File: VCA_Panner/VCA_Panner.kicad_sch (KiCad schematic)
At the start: 40 parts, among them J1 CV1, J2 Ch1_in, J3 Ch1_out, J4 CV2, J5 Ch2_in, J6 Ch2_out, SW1 SW_DPDT_x2, SW2 SW_DPDT_x2, U1 TL074, U2 AS3360, U3 TL072

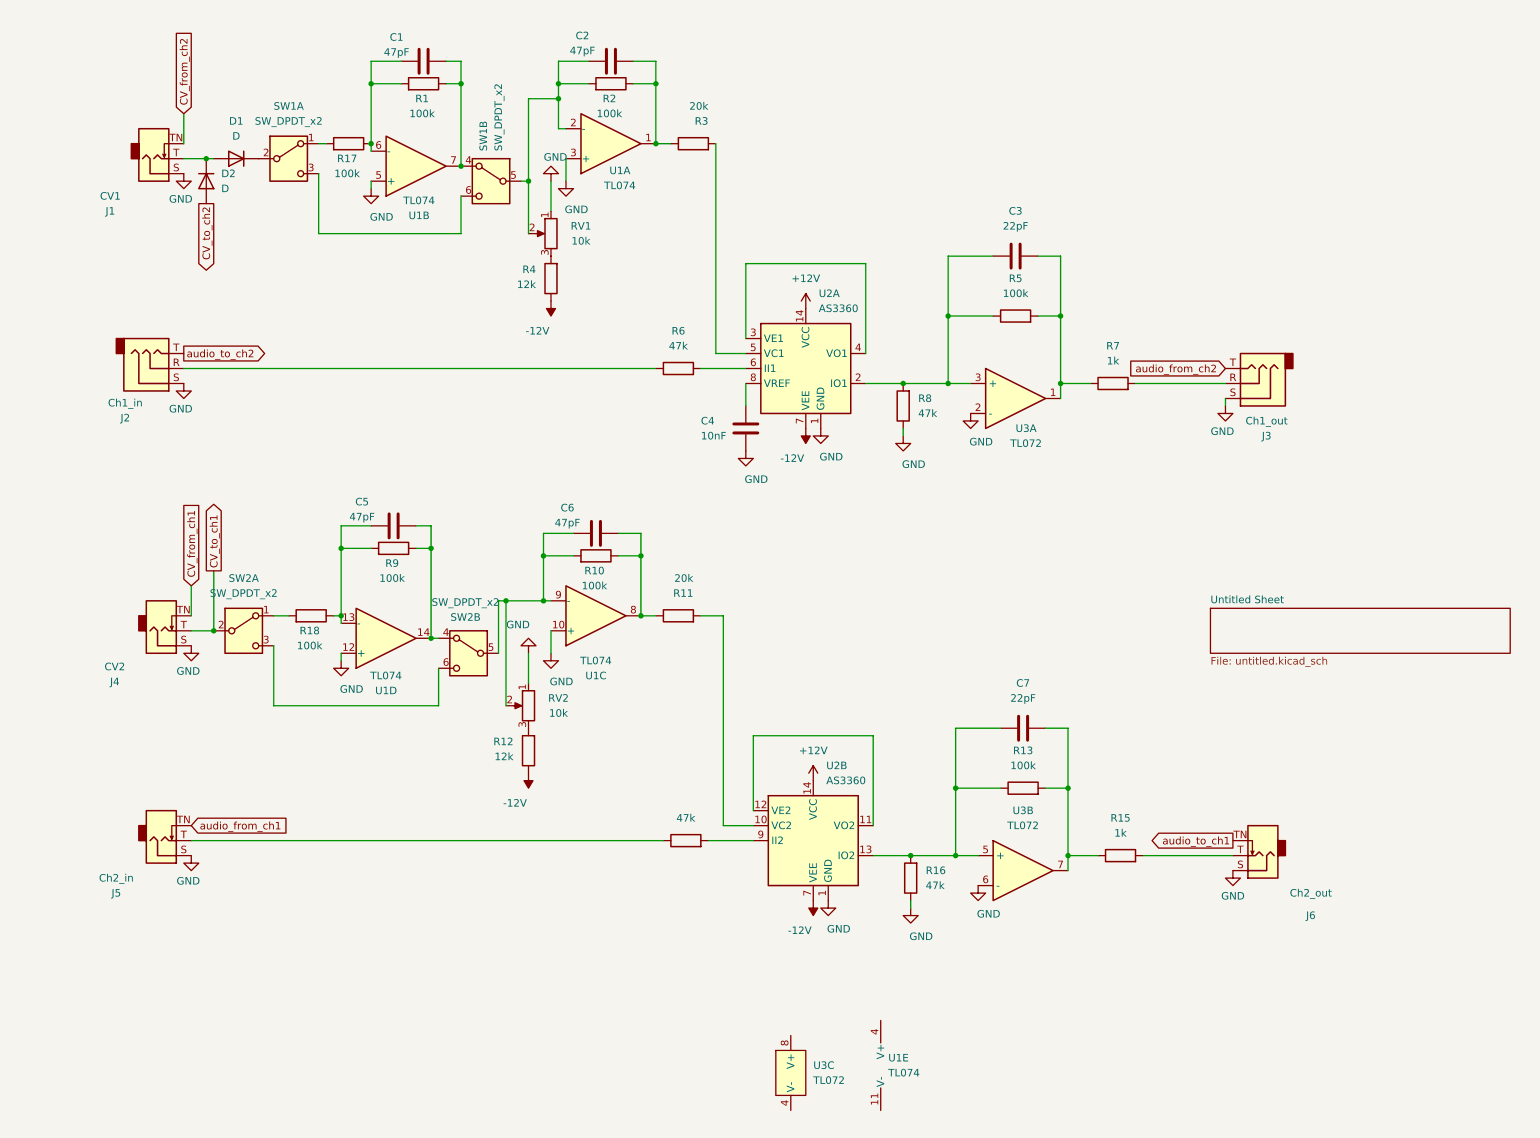
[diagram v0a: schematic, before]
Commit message: feitw bugfixes
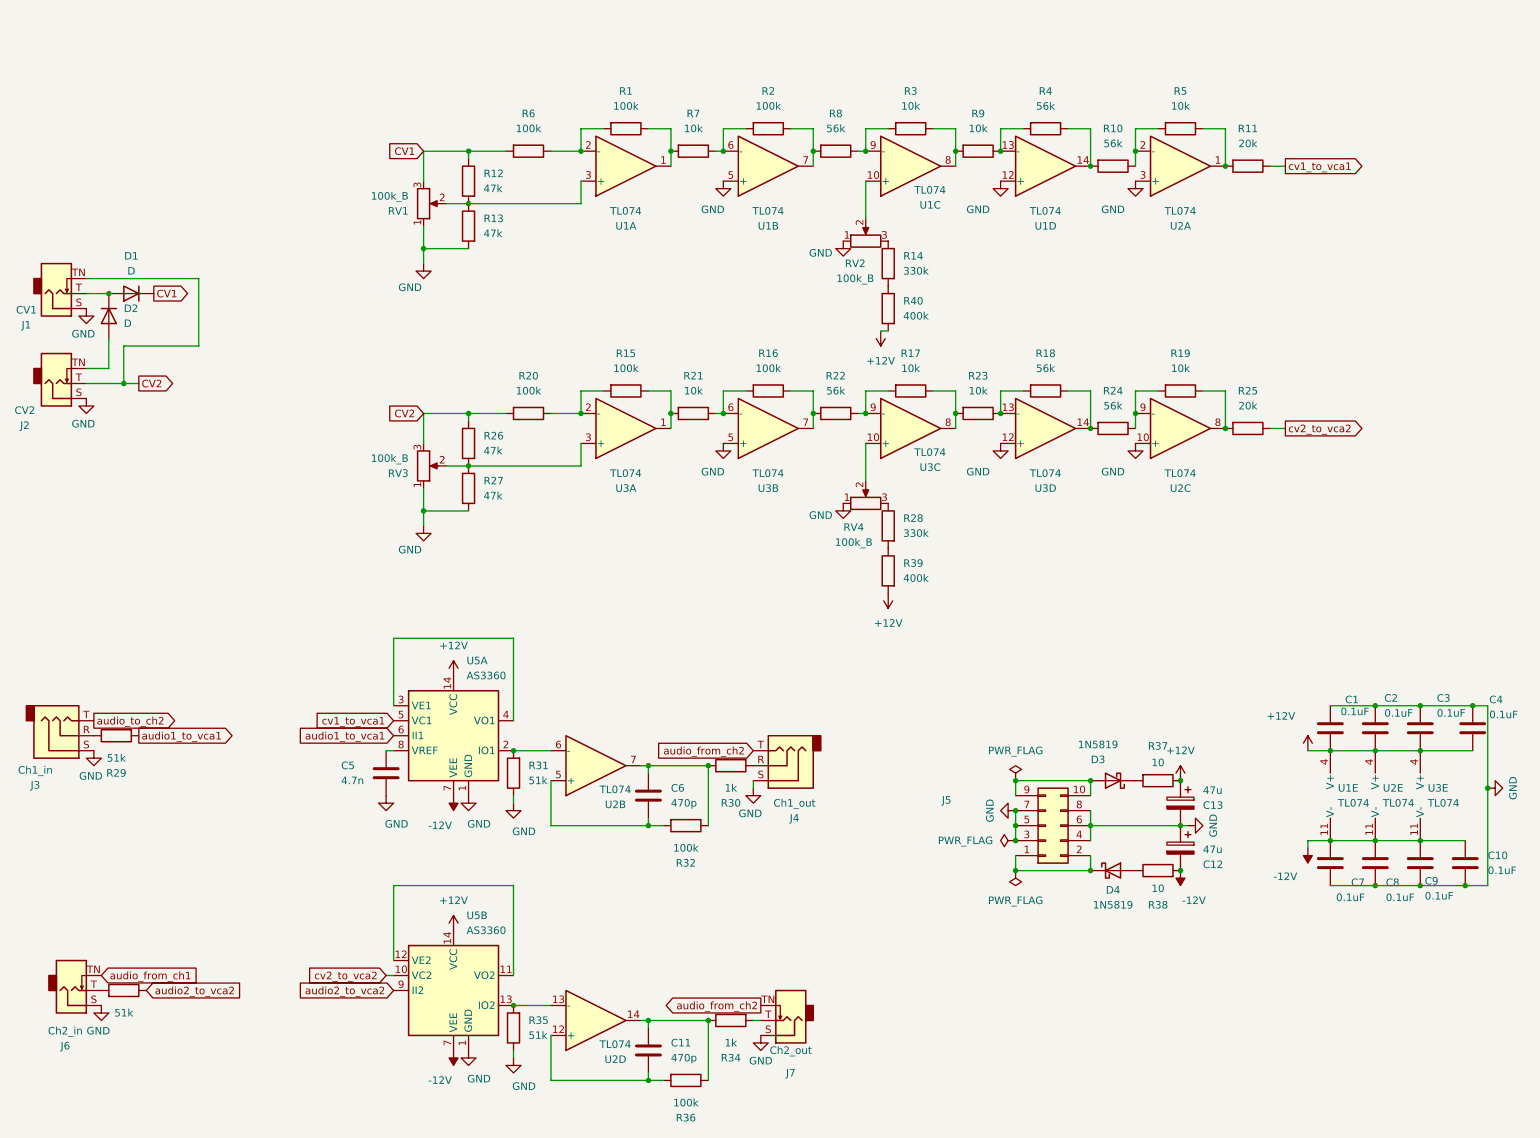
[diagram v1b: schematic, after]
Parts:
- removed C5: 47pF, symbol Device:C
- removed SW1, SW2: SW_DPDT_x2, symbol Switch:SW_DPDT_x2
- removed U3: TL072, 4ms_Package_SSOP:TSSOP-8_4.4x3mm_Pitch0.65mm, symbol PCM_4ms_IC:TL072
- added C10, C4, C8, C9: 0.1uF, Capacitor_SMD:C_0805_2012Metric_Pad1.18x1.45mm_HandSolder, symbol Device:C
- added C11: 470p, Capacitor_SMD:C_0805_2012Metric_Pad1.18x1.45mm_HandSolder, symbol Device:C
- added C12, C13: 47u, Capacitor_THT:CP_Radial_D4.0mm_P2.00mm, symbol Device:C_Polarized
- added D3, D4: 1N5819, Diode_THT:D_DO-41_SOD81_P2.54mm_Vertical_AnodeUp, symbol Diode:1N5819
- added J5: ~, mort_mix:Pins_2x05_2.54mm_TH_Europower_shrouded, symbol Connector_Generic:Conn_02x05_Odd_Even
- added R19, R21, R23, R7: 10k, Resistor_SMD:R_0805_2012Metric_Pad1.20x1.40mm_HandSolder, symbol Device:R
- added R20, R32, R36: 100k, Resistor_SMD:R_0805_2012Metric_Pad1.20x1.40mm_HandSolder, symbol Device:R
- added R22, R24, R8: 56k, Resistor_SMD:R_0805_2012Metric_Pad1.20x1.40mm_HandSolder, symbol Device:R
- added R25: 20k, Resistor_SMD:R_0805_2012Metric_Pad1.20x1.40mm_HandSolder, symbol Device:R
- added R26, R27: 47k, Resistor_SMD:R_0805_2012Metric_Pad1.20x1.40mm_HandSolder, symbol Device:R
- added R28: 330k, Resistor_SMD:R_0805_2012Metric_Pad1.20x1.40mm_HandSolder, symbol Device:R
- added R29, R33, R35: 51k, Resistor_SMD:R_0805_2012Metric_Pad1.20x1.40mm_HandSolder, symbol Device:R
- added R34: 1k, Resistor_SMD:R_0805_2012Metric_Pad1.20x1.40mm_HandSolder, symbol Device:R
- added R37, R38: 10, Resistor_SMD:R_0805_2012Metric_Pad1.20x1.40mm_HandSolder, symbol Device:R
- added R39, R40: 400k, Resistor_SMD:R_0805_2012Metric_Pad1.20x1.40mm_HandSolder, symbol Device:R
- added RV3, RV4: 100k_B, mort_mix:Potentiometer_Alpha_RD901F-40-00D_Single_Vertical_withhole, symbol Device:R_Potentiometer
- added U2, U3: TL074, Package_SO:SO-14_3.9x8.65mm_P1.27mm, symbol Amplifier_Operational:TL074
- C1, C2: value 47pF -> 0.1uF; footprint (none) -> Capacitor_SMD:C_0805_2012Metric_Pad1.18x1.45mm_HandSolder
- C3, C7: value 22pF -> 0.1uF; footprint (none) -> Capacitor_SMD:C_0805_2012Metric_Pad1.18x1.45mm_HandSolder
- C5: renamed from C4; value 10nF -> 4.7n; footprint (none) -> Capacitor_SMD:C_0805_2012Metric_Pad1.18x1.45mm_HandSolder
- C6: value 47pF -> 470p; footprint (none) -> Capacitor_SMD:C_0805_2012Metric_Pad1.18x1.45mm_HandSolder
- D1, D2: footprint (none) -> Diode_SMD:D_0805_2012Metric_Pad1.15x1.40mm_HandSolder
- J1: footprint (none) -> mort_mix:PJ398SM
- J2: renamed from J4; footprint (none) -> mort_mix:PJ398SM
- J3: renamed from J2; footprint (none) -> mort_mix:Jack_3.5mm_QingPu_WQP-PJ366ST_Vertical
- J4: renamed from J3; footprint (none) -> mort_mix:Jack_3.5mm_QingPu_WQP-PJ366ST_Vertical
- J6: renamed from J5; footprint (none) -> mort_mix:PJ398SM
- J7: renamed from J6; footprint (none) -> mort_mix:PJ398SM
- R1, R11, R2: footprint (none) -> Resistor_SMD:R_0805_2012Metric_Pad1.20x1.40mm_HandSolder
- R10, R18: value 100k -> 56k; footprint (none) -> Resistor_SMD:R_0805_2012Metric_Pad1.20x1.40mm_HandSolder
- R12: value 12k -> 47k; footprint (none) -> Resistor_SMD:R_0805_2012Metric_Pad1.20x1.40mm_HandSolder
- R13: value 100k -> 47k; footprint (none) -> Resistor_SMD:R_0805_2012Metric_Pad1.20x1.40mm_HandSolder
- R14: value 47k -> 330k; footprint (none) -> Resistor_SMD:R_0805_2012Metric_Pad1.20x1.40mm_HandSolder
- R15: value 1k -> 100k; footprint (none) -> Resistor_SMD:R_0805_2012Metric_Pad1.20x1.40mm_HandSolder
- R16, R6: value 47k -> 100k; footprint (none) -> Resistor_SMD:R_0805_2012Metric_Pad1.20x1.40mm_HandSolder
- R17, R5, R9: value 100k -> 10k; footprint (none) -> Resistor_SMD:R_0805_2012Metric_Pad1.20x1.40mm_HandSolder
- R3: value 20k -> 10k; footprint (none) -> Resistor_SMD:R_0805_2012Metric_Pad1.20x1.40mm_HandSolder
- R30: renamed from R7; footprint (none) -> Resistor_SMD:R_0805_2012Metric_Pad1.20x1.40mm_HandSolder
- R31: renamed from R8; value 47k -> 51k; footprint (none) -> Resistor_SMD:R_0805_2012Metric_Pad1.20x1.40mm_HandSolder
- R4: value 12k -> 56k; footprint (none) -> Resistor_SMD:R_0805_2012Metric_Pad1.20x1.40mm_HandSolder
- RV1, RV2: value 10k -> 100k_B; footprint (none) -> mort_mix:Potentiometer_Alpha_RD901F-40-00D_Single_Vertical_withhole
- U1: footprint (none) -> Package_SO:SO-14_3.9x8.65mm_P1.27mm
- U5: renamed from U2; footprint (none) -> Package_SO:SOIC-16_3.9x9.9mm_P1.27mm
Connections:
- net CV_to_ch1 is gone; now on net CV2: J2.T
- net CV_to_ch2 is gone; now on an unnamed net: D2.2 (A)
- net audio_to_ch1 is gone; now on net audio_from_ch2: J7.TN
- net +12V: now also C1.1, C2.1, C3.1, U1.4 (V+), C13.1, C4.2, R37.1, R39.2, R40.2, U2.4 (V+), U3.4 (V+)
- net -12V: now also C7.2, U1.11 (V-), C10.2, C12.2, C8.2, C9.2, R38.2, U2.11 (V-), U3.11 (V-); no longer R12.1, R4.1
- net GND: now also C1.2, C2.2, C3.2, C7.1, R13.2, C10.1, C12.1, C13.2, C4.1, C8.1, C9.1, J5.3 (Pin_3), J5.4 (Pin_4), J5.5 (Pin_5), J5.6 (Pin_6), J5.7 (Pin_7), J5.8 (Pin_8), R27.2, R35.1, RV3.1, RV4.1, U2.10 (+), U2.3 (+), U3.12 (+), U3.5 (+); no longer R16.1, U1.10 (+), U1.3 (+)
- net at R31.2, U5.2 (IO1): now also U2.6 (-); no longer C3.1, R5.1
- net CV1: now reaches D1.1 (K)
- net CV1: now also R12.1, R6.2, RV1.3
- net at R12.2: now also R13.1, RV1.2, U1.3 (+); no longer RV2.3
- net at R18.2: now also R23.1, U3.13 (-)
- net at R14.1: now also RV2.3; no longer J6.T
- net at R6.1: now also R1.2, U1.2 (-); no longer J3.R
- net audio1_to_vca1: now reaches U5.6 (II1)
- net audio1_to_vca1: now also R29.2; no longer R6.2
- net at R11.2: now also R5.1, U2.1; no longer U5.10 (VC2)
- net at R9.1: now also R4.2, U1.13 (-); no longer U1.14
- net at R3.2: now also U1.9 (-), R8.1; no longer U5.5 (VC1)
- net at R17.2: now also R22.1, U3.9 (-)
- net at R15.2: now also R20.1, U3.2 (-); no longer J7.T
- net at R14.2: now also R40.1; no longer U5.9 (II2)
- net CV_from_ch1: no longer names the net of J2.TN
- net CV_from_ch2 renamed CV2
- net CV2: now also R20.2, R26.1, RV3.3
- new net: R3.1, R9.2, U1.8
- new net: RV2.2, U1.10 (+)
- new net: R15.1, R21.2, U3.1
- new net: R26.2, R27.1, RV3.2, U3.3 (+)
- new net: R18.1, R24.2, U3.14
- new net: R10.1, R5.2, U2.2 (-)
- new net: R10.2, R4.1, U1.14
- new net: D4.2 (A), R38.1
- new net: R16.1, R22.2, U3.7
- new net: R16.2, R21.1, U3.6 (-)
- new net: C11.2, R34.1, R36.1, U2.14
- new net: C11.1, R36.2, U2.12 (+)
- new net: R19.2, R24.1, U2.9 (-)
- new net: D3.1 (K), R37.2
- new net: C6.1, R32.2, U2.5 (+)
- new net: C6.2, R30.1, R32.1, U2.7
- new net: R28.1, RV4.3
- new net: R28.2, R39.1
- new net: D3.2 (A), J5.10 (Pin_10), J5.9 (Pin_9)
- new net: J7.T, R34.2
- new net: R1.1, R7.2, U1.1
- new net: R17.1, R23.2, U3.8
- new net: R35.2, U2.13 (-), U5.13 (IO2)
- new net: RV4.2, U3.10 (+)
- new net: J6.T, R33.2
- new net: R2.1, R8.2, U1.7
- new net: R19.1, R25.2, U2.8
- new net: J3.R, R29.1
- new net: D4.1 (K), J5.1 (Pin_1), J5.2 (Pin_2)
- new net: R2.2, R7.1, U1.6 (-)
- new net audio2_to_vca2: R33.1, U5.9 (II2)
- new net cv1_to_vca1: R11.1, U5.5 (VC1)
- new net cv2_to_vca2: R25.1, U5.10 (VC2)
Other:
- removed sheet Untitled Sheet
- company: (none) -> Clandestine Circutry
- title: (none) -> VCA_Panner
- moved on the sheet: C5, D1, D2, J1, J2, J3, J4, J6, J7, R30, R31, U5A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
